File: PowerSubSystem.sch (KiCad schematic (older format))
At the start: 14 parts

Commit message: FOUR LAYER BOARD CHANGE. We still need to adapt the other subsystems for four layers
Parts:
- gave numbers to parts that had none: 2
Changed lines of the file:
@@
 5Vin+ Comes from the 5V output \nof the beaglebone. The one \nthat is connected to the 12V \ninput.
 $Comp
-L pwr_BeagleBone:LM3671 U?
+L pwr_BeagleBone:LM3671 U401
 U 1 1 613D6B2B
 P 3650 6150
-F 0 "U?" H 3650 6250 50  0000 C CNN
+F 0 "U401" H 3650 6250 50  0000 C CNN
 F 1 "LM3671" H 3650 6150 50  0000 C CNN
 F 2 "Package_TO_SOT_SMD:SOT-23-5" H 3650 6150 50  0001 C CNN
@@
 	3200 6500 3200 6800
 $Comp
-L Device:L_Small L?
+L Device:L_Small L401
 U 1 1 613E2221
 P 4200 6300
-F 0 "L?" V 4385 6300 50  0000 C CNN
+F 0 "L401" V 4385 6300 50  0000 C CNN
 F 1 "2.2uH" V 4294 6300 50  0000 C CNN
 F 2 "Inductor_SMD:L_1210_3225Metric" H 4200 6300 50  0001 C CNN

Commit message: Recovered the .lib for flash symbol. Relinked in schematic
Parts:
- C401, C402, C404, C405, C406, C408, C409, C410: symbol Device:C -> BeagleBone-Black-Cape-rescue:C-Device
- C403, C407: symbol Device:C_Small -> BeagleBone-Black-Cape-rescue:C_Small-Device
- FB401: symbol Device:Ferrite_Bead_Small -> BeagleBone-Black-Cape-rescue:Ferrite_Bead_Small-Device
- L401: symbol Device:L_Small -> BeagleBone-Black-Cape-rescue:L_Small-Device
- L402: symbol pspice:INDUCTOR -> BeagleBone-Black-Cape-rescue:INDUCTOR-pspice
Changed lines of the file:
@@
 $EndComp
 $Comp
-L Device:C_Small C403
+L BeagleBone-Black-Cape-rescue:C_Small-Device C403
 U 1 1 613D8B5E
 P 3000 6550
@@
 	3200 6500 3200 6800
 $Comp
-L Device:L_Small L401
+L BeagleBone-Black-Cape-rescue:L_Small-Device L401
 U 1 1 613E2221
 P 4200 6300
@@
 	4400 6500 4400 6300
 $Comp
-L power:GND #PWR0404
+L BeagleBone-Black-Cape-rescue:GND-power #PWR0404
 U 1 1 613E4C24
 P 3000 6900
@@
 	3000 6900 3000 6800
 $Comp
-L Device:C_Small C407
+L BeagleBone-Black-Cape-rescue:C_Small-Device C407
 U 1 1 613E66FD
 P 4650 6550
@@
 $EndComp
 $Comp
-L power:GND #PWR0408
+L BeagleBone-Black-Cape-rescue:GND-power #PWR0408
 U 1 1 613EB575
 P 4650 6900
@@
 VDDR
 $Comp
-L Device:C C402
+L BeagleBone-Black-Cape-rescue:C-Device C402
 U 1 1 614ACFF1
 P 2800 2950
@@
 $EndComp
 $Comp
-L Device:C C401
+L BeagleBone-Black-Cape-rescue:C-Device C401
 U 1 1 614AD67F
 P 2300 2950
@@
 $EndComp
 $Comp
-L Device:C C409
+L BeagleBone-Black-Cape-rescue:C-Device C409
 U 1 1 614ADB54
 P 8450 2950
@@
 $EndComp
 $Comp
-L Device:C C406
+L BeagleBone-Black-Cape-rescue:C-Device C406
 U 1 1 614ADE06
 P 4350 2950
@@
 $EndComp
 $Comp
-L Device:C C404
+L BeagleBone-Black-Cape-rescue:C-Device C404
 U 1 1 614ADFDD
 P 3300 2950
@@
 $EndComp
 $Comp
-L Device:C C410
+L BeagleBone-Black-Cape-rescue:C-Device C410
 U 1 1 614AE392
 P 8950 2950
@@
 $EndComp
 $Comp
-L Device:C C405
+L BeagleBone-Black-Cape-rescue:C-Device C405
 U 1 1 614AE569
 P 3850 2950
@@
 $EndComp
 $Comp
-L Device:C C408
+L BeagleBone-Black-Cape-rescue:C-Device C408
 U 1 1 614AE740
 P 7600 2950
@@
 $EndComp
 $Comp
-L pspice:INDUCTOR L402
+L BeagleBone-Black-Cape-rescue:INDUCTOR-pspice L402
 U 1 1 614B2435
 P 7050 2800
@@
 $EndComp
 $Comp
-L power:GND #PWR0401
+L BeagleBone-Black-Cape-rescue:GND-power #PWR0401
 U 1 1 614B60EB
 P 2300 3100
@@
 $EndComp
 $Comp
-L power:GND #PWR0403
+L BeagleBone-Black-Cape-rescue:GND-power #PWR0403
 U 1 1 614B633D
 P 2800 3100
@@
 $EndComp
 $Comp
-L power:GND #PWR0405
+L BeagleBone-Black-Cape-rescue:GND-power #PWR0405
 U 1 1 614B6607
 P 3300 3100
@@
 $EndComp
 $Comp
-L power:GND #PWR0406
+L BeagleBone-Black-Cape-rescue:GND-power #PWR0406
 U 1 1 614B68D5
 P 3850 3100
@@
 $EndComp
 $Comp
-L power:GND #PWR0407
+L BeagleBone-Black-Cape-rescue:GND-power #PWR0407
 U 1 1 614B6CF8
 P 4350 3100
@@
 $EndComp
 $Comp
-L power:GND #PWR0409
+L BeagleBone-Black-Cape-rescue:GND-power #PWR0409
 U 1 1 614B73B7
 P 7600 3100
@@
 $EndComp
 $Comp
-L power:GND #PWR0410
+L BeagleBone-Black-Cape-rescue:GND-power #PWR0410
 U 1 1 614B76A1
 P 8450 3100
@@
 $EndComp
 $Comp
-L power:GND #PWR0411
+L BeagleBone-Black-Cape-rescue:GND-power #PWR0411
 U 1 1 614B7948
 P 8950 3100
@@
 MCU_VDD
 $Comp
-L Device:Ferrite_Bead_Small FB401
+L BeagleBone-Black-Cape-rescue:Ferrite_Bead_Small-Device FB401
 U 1 1 614B96C9
 P 2000 2800

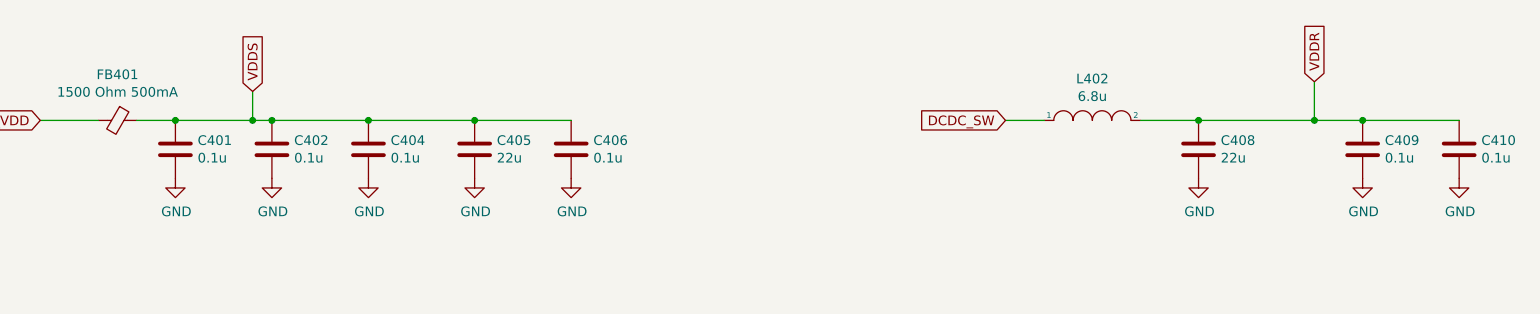
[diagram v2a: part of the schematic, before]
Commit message: slow and steady wins the race. Zach read the ZACH READ ME.txt
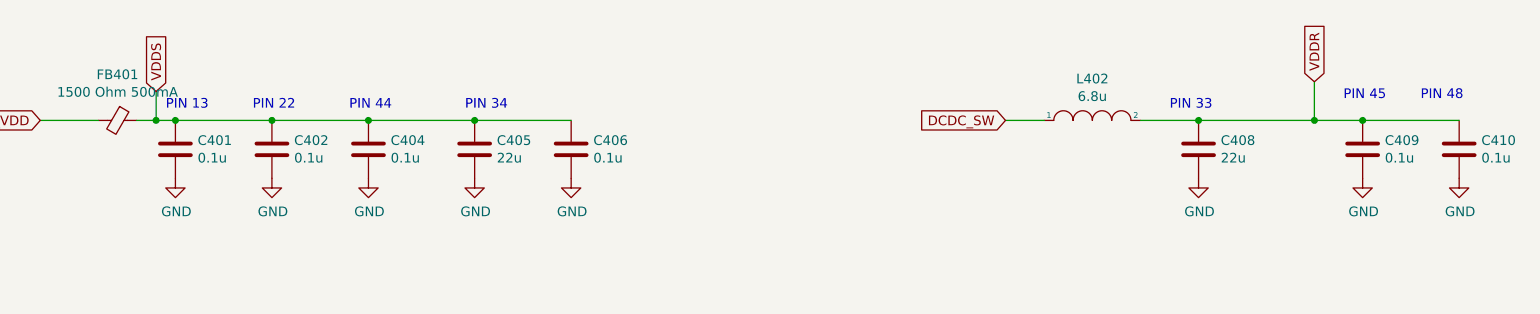
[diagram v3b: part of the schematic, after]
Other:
- note added: "PIN 13"
- note added: "PIN 22"
- note added: "PIN 33"
- note added: "PIN 34"
- note added: "PIN 44\n"
- note added: "PIN 45"
- note added: "PIN 48\n"
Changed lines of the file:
@@
 Wire Wire Line
 	2650 6300 3000 6300
-Text GLabel 2700 2650 1    50   Input ~ 0
+Text GLabel 2200 2650 1    50   Input ~ 0
 VDDS
 Text GLabel 8200 2600 1    50   Input ~ 0
@@
 Wire Wire Line
 	8200 2800 8450 2800
-Wire Wire Line
-	2300 2800 2700 2800
 Connection ~ 2800 2800
 Wire Wire Line
@@
 	3850 2800 4350 2800
 Wire Wire Line
-	2700 2650 2700 2800
-Connection ~ 2700 2800
-Wire Wire Line
-	2700 2800 2800 2800
+	2200 2650 2200 2800
 Text GLabel 1600 2800 0    50   Input ~ 0
 MCU_VDD
@@
 $EndComp
 Wire Wire Line
-	2100 2800 2300 2800
+	2100 2800 2200 2800
 Connection ~ 2300 2800
 Wire Wire Line
 	1600 2800 1900 2800
+Text Notes 2700 2750 0    50   ~ 0
+PIN 22
+Connection ~ 2200 2800
+Wire Wire Line
+	2200 2800 2300 2800
+Wire Wire Line
+	2300 2800 2800 2800
+Text Notes 2250 2750 0    50   ~ 0
+PIN 13
+Text Notes 3200 2750 0    50   ~ 0
+PIN 44\n
+Text Notes 3800 2750 0    50   ~ 0
+PIN 34
+Text Notes 7450 2750 0    50   ~ 0
+PIN 33
+Text Notes 8350 2700 0    50   ~ 0
+PIN 45
+Text Notes 8750 2700 0    50   ~ 0
+PIN 48\n
 $EndSCHEMATC

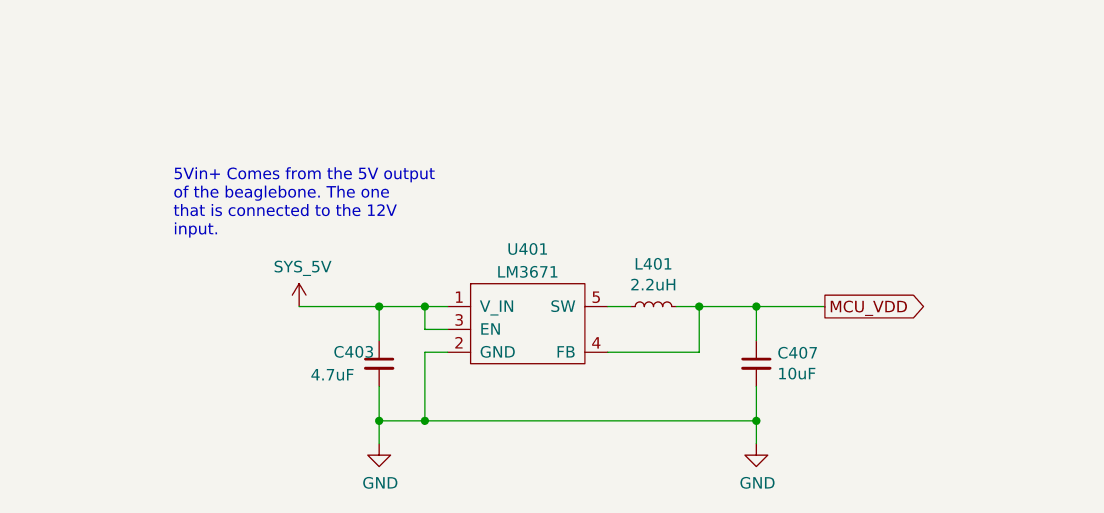
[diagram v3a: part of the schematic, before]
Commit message: sync push so zach can work
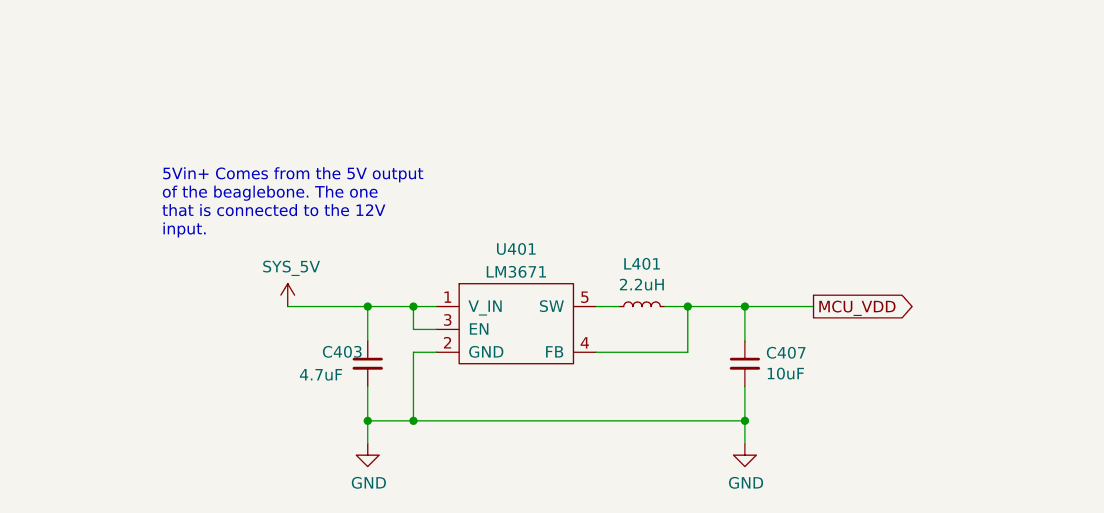
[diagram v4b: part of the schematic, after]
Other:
- moved on the sheet: C403, C407, L401, U401
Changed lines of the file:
@@
 Comment4 ""
 $EndDescr
-Text Notes 2100 6000 0    50   ~ 0
+Text Notes 2050 6000 0    50   ~ 0
 5Vin+ Comes from the 5V output \nof the beaglebone. The one \nthat is connected to the 12V \ninput.
 $Comp
 L pwr_BeagleBone:LM3671 U401
 U 1 1 613D6B2B
-P 3650 6150
-F 0 "U401" H 3650 6250 50  0000 C CNN
-F 1 "LM3671" H 3650 6150 50  0000 C CNN
-F 2 "Package_TO_SOT_SMD:SOT-23-5" H 3650 6150 50  0001 C CNN
-F 3 "https://www.ti.com/lit/ds/symlink/lm3671.pdf?HQS=dis-mous-null-mousermode-dsf-pf-null-wwe&ts=1631307057229&ref_url=https%253A%252F%252Fwww.mouser.com%252F" H 3650 6150 50  0001 C CNN
-	1    3650 6150
+P 3600 6150
+F 0 "U401" H 3600 6250 50  0000 C CNN
+F 1 "LM3671" H 3600 6150 50  0000 C CNN
+F 2 "Package_TO_SOT_SMD:SOT-23-5" H 3600 6150 50  0001 C CNN
+F 3 "https://www.ti.com/lit/ds/symlink/lm3671.pdf?HQS=dis-mous-null-mousermode-dsf-pf-null-wwe&ts=1631307057229&ref_url=https%253A%252F%252Fwww.mouser.com%252F" H 3600 6150 50  0001 C CNN
+	1    3600 6150
 	1    0    0    -1
 $EndComp
@@
 L BeagleBone-Black-Cape-rescue:C_Small-Device C403
 U 1 1 613D8B5E
-P 3000 6550
-F 0 "C403" H 2800 6600 50  0000 L CNN
-F 1 "4.7uF" H 2700 6500 50  0000 L CNN
-F 2 "Capacitor_SMD:C_0805_2012Metric" H 3000 6550 50  0001 C CNN
-F 3 "https://www.mouser.com/datasheet/2/396/mlcc02_e-1307760.pdf" H 3000 6550 50  0001 C CNN
-	1    3000 6550
+P 2950 6550
+F 0 "C403" H 2750 6600 50  0000 L CNN
+F 1 "4.7uF" H 2650 6500 50  0000 L CNN
+F 2 "Capacitor_SMD:C_0805_2012Metric" H 2950 6550 50  0001 C CNN
+F 3 "https://www.mouser.com/datasheet/2/396/mlcc02_e-1307760.pdf" H 2950 6550 50  0001 C CNN
+	1    2950 6550
 	1    0    0    -1
 $EndComp
 Wire Wire Line
-	3000 6450 3000 6300
+	2950 6450 2950 6300
 Wire Wire Line
-	3000 6650 3000 6800
-Connection ~ 3000 6800
+	2950 6650 2950 6800
+Connection ~ 2950 6800
 Wire Wire Line
-	3300 6400 3200 6400
+	3250 6400 3150 6400
 Wire Wire Line
-	3200 6400 3200 6300
+	3150 6400 3150 6300
 Wire Wire Line
-	3200 6300 3300 6300
+	3150 6300 3250 6300
 Wire Wire Line
-	3300 6500 3200 6500
+	3250 6500 3150 6500
 Wire Wire Line
-	3200 6500 3200 6800
+	3150 6500 3150 6800
 $Comp
 L BeagleBone-Black-Cape-rescue:L_Small-Device L401
 U 1 1 613E2221
-P 4200 6300
-F 0 "L401" V 4385 6300 50  0000 C CNN
-F 1 "2.2uH" V 4294 6300 50  0000 C CNN
-F 2 "Inductor_SMD:L_1210_3225Metric" H 4200 6300 50  0001 C CNN
-F 3 "~https://www.mouser.com/datasheet/2/54/cm322522-777598.pdf" H 4200 6300 50  0001 C CNN
-	1    4200 6300
+P 4150 6300
+F 0 "L401" V 4335 6300 50  0000 C CNN
+F 1 "2.2uH" V 4244 6300 50  0000 C CNN
+F 2 "Inductor_SMD:L_1210_3225Metric" H 4150 6300 50  0001 C CNN
+F 3 "~https://www.mouser.com/datasheet/2/54/cm322522-777598.pdf" H 4150 6300 50  0001 C CNN
+	1    4150 6300
 	0    -1   -1   0
 $EndComp
 Wire Wire Line
-	4000 6300 4100 6300
+	3950 6300 4050 6300
 Wire Wire Line
-	4400 6500 4400 6300
+	4350 6500 4350 6300
 $Comp
 L BeagleBone-Black-Cape-rescue:GND-power #PWR0404
 U 1 1 613E4C24
-P 3000 6900
-F 0 "#PWR0404" H 3000 6650 50  0001 C CNN
-F 1 "GND" H 3005 6727 50  0000 C CNN
-F 2 "" H 3000 6900 50  0001 C CNN
-F 3 "" H 3000 6900 50  0001 C CNN
-	1    3000 6900
+P 2950 6900
+F 0 "#PWR0404" H 2950 6650 50  0001 C CNN
+F 1 "GND" H 2955 6727 50  0000 C CNN
+F 2 "" H 2950 6900 50  0001 C CNN
+F 3 "" H 2950 6900 50  0001 C CNN
+	1    2950 6900
 	1    0    0    -1
 $EndComp
 Wire Wire Line
-	3000 6900 3000 6800
+	2950 6900 2950 6800
 $Comp
 L BeagleBone-Black-Cape-rescue:C_Small-Device C407
 U 1 1 613E66FD
-P 4650 6550
-F 0 "C407" H 4742 6596 50  0000 L CNN
-F 1 "10uF" H 4742 6505 50  0000 L CNN
-F 2 "Capacitor_SMD:C_0805_2012Metric" H 4650 6550 50  0001 C CNN
-F 3 "https://www.mouser.com/datasheet/2/396/mlcc02_e-1307760.pdf" H 4650 6550 50  0001 C CNN
-	1    4650 6550
+P 4600 6550
+F 0 "C407" H 4692 6596 50  0000 L CNN
+F 1 "10uF" H 4692 6505 50  0000 L CNN
+F 2 "Capacitor_SMD:C_0805_2012Metric" H 4600 6550 50  0001 C CNN
+F 3 "https://www.mouser.com/datasheet/2/396/mlcc02_e-1307760.pdf" H 4600 6550 50  0001 C CNN
+	1    4600 6550
 	1    0    0    -1
 $EndComp
@@
 L BeagleBone-Black-Cape-rescue:GND-power #PWR0408
 U 1 1 613EB575
-P 4650 6900
-F 0 "#PWR0408" H 4650 6650 50  0001 C CNN
-F 1 "GND" H 4655 6727 50  0000 C CNN
-F 2 "" H 4650 6900 50  0001 C CNN
-F 3 "" H 4650 6900 50  0001 C CNN
-	1    4650 6900
+P 4600 6900
+F 0 "#PWR0408" H 4600 6650 50  0001 C CNN
+F 1 "GND" H 4605 6727 50  0000 C CNN
+F 2 "" H 4600 6900 50  0001 C CNN
+F 3 "" H 4600 6900 50  0001 C CNN
+	1    4600 6900
 	1    0    0    -1
 $EndComp
-Text GLabel 4950 6300 2    50   Output ~ 0
+Text GLabel 4900 6300 2    50   Output ~ 0
 MCU_VDD
 Wire Wire Line
-	4650 6300 4650 6450
+	4600 6300 4600 6450
 Wire Wire Line
-	4400 6300 4650 6300
+	4350 6300 4600 6300
 Wire Wire Line
-	4650 6300 4950 6300
-Connection ~ 4650 6300
+	4600 6300 4900 6300
+Connection ~ 4600 6300
 Wire Wire Line
-	4650 6800 4650 6650
+	4600 6800 4600 6650
 Wire Wire Line
-	4650 6900 4650 6800
-Connection ~ 4650 6800
+	4600 6900 4600 6800
+Connection ~ 4600 6800
 Wire Wire Line
-	3000 6800 3200 6800
+	2950 6800 3150 6800
 Wire Wire Line
-	3200 6300 3000 6300
-Connection ~ 3200 6300
-Connection ~ 3000 6300
+	3150 6300 2950 6300
+Connection ~ 3150 6300
+Connection ~ 2950 6300
 Wire Wire Line
-	4300 6300 4400 6300
-Connection ~ 4400 6300
+	4250 6300 4350 6300
+Connection ~ 4350 6300
 Wire Wire Line
-	4000 6500 4400 6500
+	3950 6500 4350 6500
 Wire Wire Line
-	3200 6800 4650 6800
-Connection ~ 3200 6800
+	3150 6800 4600 6800
+Connection ~ 3150 6800
 $Comp
 L pwr_BeagleBone:SYS_5V #PWR0402
 U 1 1 614A8F35
-P 2650 6300
-F 0 "#PWR0402" H 2650 6150 50  0001 C CNN
-F 1 "SYS_5V" H 2665 6473 50  0000 C CNN
-F 2 "" H 2650 6300 60  0000 C CNN
-F 3 "" H 2650 6300 60  0000 C CNN
-	1    2650 6300
+P 2600 6300
+F 0 "#PWR0402" H 2600 6150 50  0001 C CNN
+F 1 "SYS_5V" H 2615 6473 50  0000 C CNN
+F 2 "" H 2600 6300 60  0000 C CNN
+F 3 "" H 2600 6300 60  0000 C CNN
+	1    2600 6300
 	1    0    0    -1
 $EndComp
 Wire Wire Line
-	2650 6300 3000 6300
+	2600 6300 2950 6300
 Text GLabel 2200 2650 1    50   Input ~ 0
 VDDS

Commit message: Massive PCB/Schematic Update
The PCB has been completed, and the schematic has been updated to have the correct footprints
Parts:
- C401, C402, C405, C406: footprint Capacitor_SMD:C_0805_2012Metric_Pad1.18x1.45mm_HandSolder -> Capacitor_SMD:C_0402_1005Metric_Pad0.74x0.62mm_HandSolder
- L402: footprint Inductor_SMD:L_0805_2012Metric_Pad1.05x1.20mm_HandSolder -> Inductor_SMD:L_0402_1005Metric_Pad0.77x0.64mm_HandSolder
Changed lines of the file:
@@
 F 0 "C402" H 2915 2996 50  0000 L CNN
 F 1 "0.1u" H 2915 2905 50  0000 L CNN
-F 2 "Capacitor_SMD:C_0805_2012Metric_Pad1.18x1.45mm_HandSolder" H 2838 2800 50  0001 C CNN
+F 2 "Capacitor_SMD:C_0402_1005Metric_Pad0.74x0.62mm_HandSolder" H 2838 2800 50  0001 C CNN
 F 3 "~" H 2800 2950 50  0001 C CNN
 	1    2800 2950
@@
 F 0 "C401" H 2415 2996 50  0000 L CNN
 F 1 "0.1u" H 2415 2905 50  0000 L CNN
-F 2 "Capacitor_SMD:C_0805_2012Metric_Pad1.18x1.45mm_HandSolder" H 2338 2800 50  0001 C CNN
+F 2 "Capacitor_SMD:C_0402_1005Metric_Pad0.74x0.62mm_HandSolder" H 2338 2800 50  0001 C CNN
 F 3 "~" H 2300 2950 50  0001 C CNN
 	1    2300 2950
@@
 F 0 "C406" H 4465 2996 50  0000 L CNN
 F 1 "0.1u" H 4465 2905 50  0000 L CNN
-F 2 "Capacitor_SMD:C_0805_2012Metric_Pad1.18x1.45mm_HandSolder" H 4388 2800 50  0001 C CNN
+F 2 "Capacitor_SMD:C_0402_1005Metric_Pad0.74x0.62mm_HandSolder" H 4388 2800 50  0001 C CNN
 F 3 "~" H 4350 2950 50  0001 C CNN
 	1    4350 2950
@@
 F 0 "C405" H 3965 2996 50  0000 L CNN
 F 1 "22u" H 3965 2905 50  0000 L CNN
-F 2 "Capacitor_SMD:C_0805_2012Metric_Pad1.18x1.45mm_HandSolder" H 3888 2800 50  0001 C CNN
+F 2 "Capacitor_SMD:C_0402_1005Metric_Pad0.74x0.62mm_HandSolder" H 3888 2800 50  0001 C CNN
 F 3 "~" H 3850 2950 50  0001 C CNN
 	1    3850 2950
@@
 F 0 "L402" H 7050 3015 50  0000 C CNN
 F 1 "6.8u" H 7050 2924 50  0000 C CNN
-F 2 "Inductor_SMD:L_0805_2012Metric_Pad1.05x1.20mm_HandSolder" H 7050 2800 50  0001 C CNN
+F 2 "Inductor_SMD:L_0402_1005Metric_Pad0.77x0.64mm_HandSolder" H 7050 2800 50  0001 C CNN
 F 3 "~" H 7050 2800 50  0001 C CNN
 	1    7050 2800

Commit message: Zach once over, resized some components, connected VDDS pins
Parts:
- C404: footprint Capacitor_SMD:C_0805_2012Metric_Pad1.18x1.45mm_HandSolder -> Capacitor_SMD:C_0402_1005Metric_Pad0.74x0.62mm_HandSolder
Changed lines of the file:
@@
 F 0 "C404" H 3415 2996 50  0000 L CNN
 F 1 "0.1u" H 3415 2905 50  0000 L CNN
-F 2 "Capacitor_SMD:C_0805_2012Metric_Pad1.18x1.45mm_HandSolder" H 3338 2800 50  0001 C CNN
+F 2 "Capacitor_SMD:C_0402_1005Metric_Pad0.74x0.62mm_HandSolder" H 3338 2800 50  0001 C CNN
 F 3 "~" H 3300 2950 50  0001 C CNN
 	1    3300 2950
